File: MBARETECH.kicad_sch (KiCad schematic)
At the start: 48 parts, among them J10 Conn_01x03, J11 Conn_01x03, J17 Conn_01x03, J18 Conn_01x03, J19 TERMINAL DRIVER, J3 XT60-M, J7 Conn_01x03, J8 Conn_01x03, J9 Conn_01x03, SW1 SW_SPDT, SW2 SW_DIP_x04, SW3 SW_SPDT, SW5 SW_SPST, U2 ESP32-S3-DevKitC

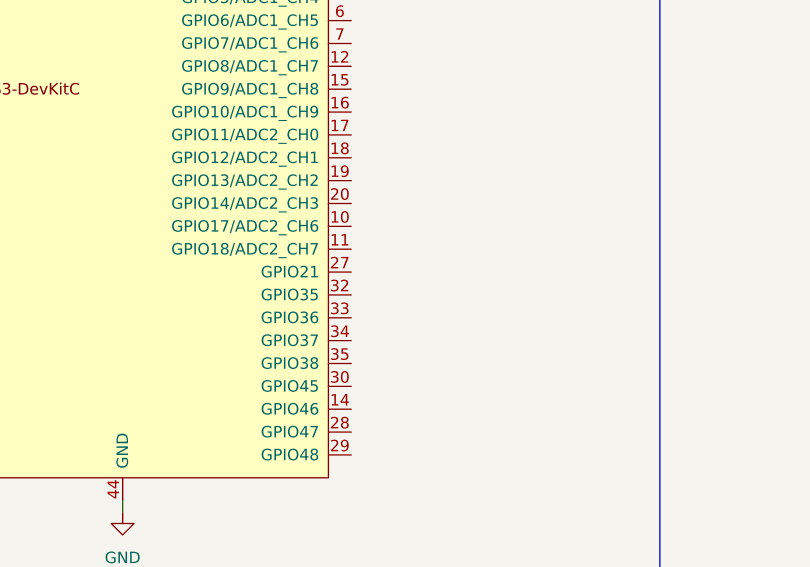
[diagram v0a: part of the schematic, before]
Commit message: test branch
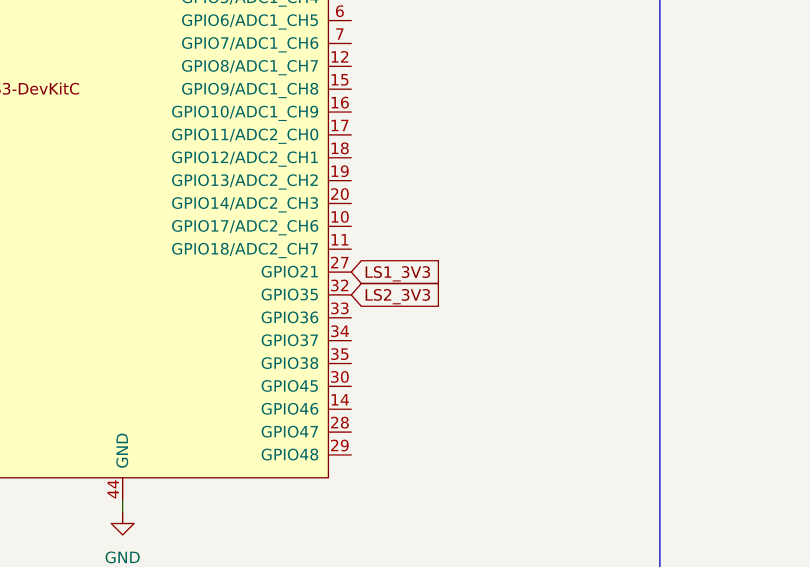
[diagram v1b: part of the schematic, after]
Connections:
- net LS1_3V3: now also U2.27 (GPIO21)
- net LS2_3V3: now also U2.32 (GPIO35)
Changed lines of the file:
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@@
+		)
+	)
+	(global_label "LS1_3V3"
+		(shape input)
+		(at 111.76 110.49 0)
+		(fields_autoplaced yes)
+		(effects
+			(font
+				(size 1.27 1.27)
+			)
+			(justify left)
+		)
+		(property "Intersheetrefs" "${INTERSHEET_REFS}"
+			(at 122.6675 110.49 0)
+			(effects
+				(font
+					(size 1.27 1.27)
+				)
+				(justify left)
+				(hide yes)
+			)
+		)
+	)
+	(global_label "LS2_3V3"
+		(shape input)
+		(at 111.76 113.03 0)
+		(fields_autoplaced yes)
+		(effects
+			(font
+				(size 1.27 1.27)
+			)
+			(justify left)
+		)
+		(property "Intersheetrefs" "${INTERSHEET_REFS}"
+			(at 122.6675 113.03 0)
+			(effects
+				(font
+					(size 1.27 1.27)
+				)
+				(justify left)
+				(hide yes)
+			)
 		)
 	)

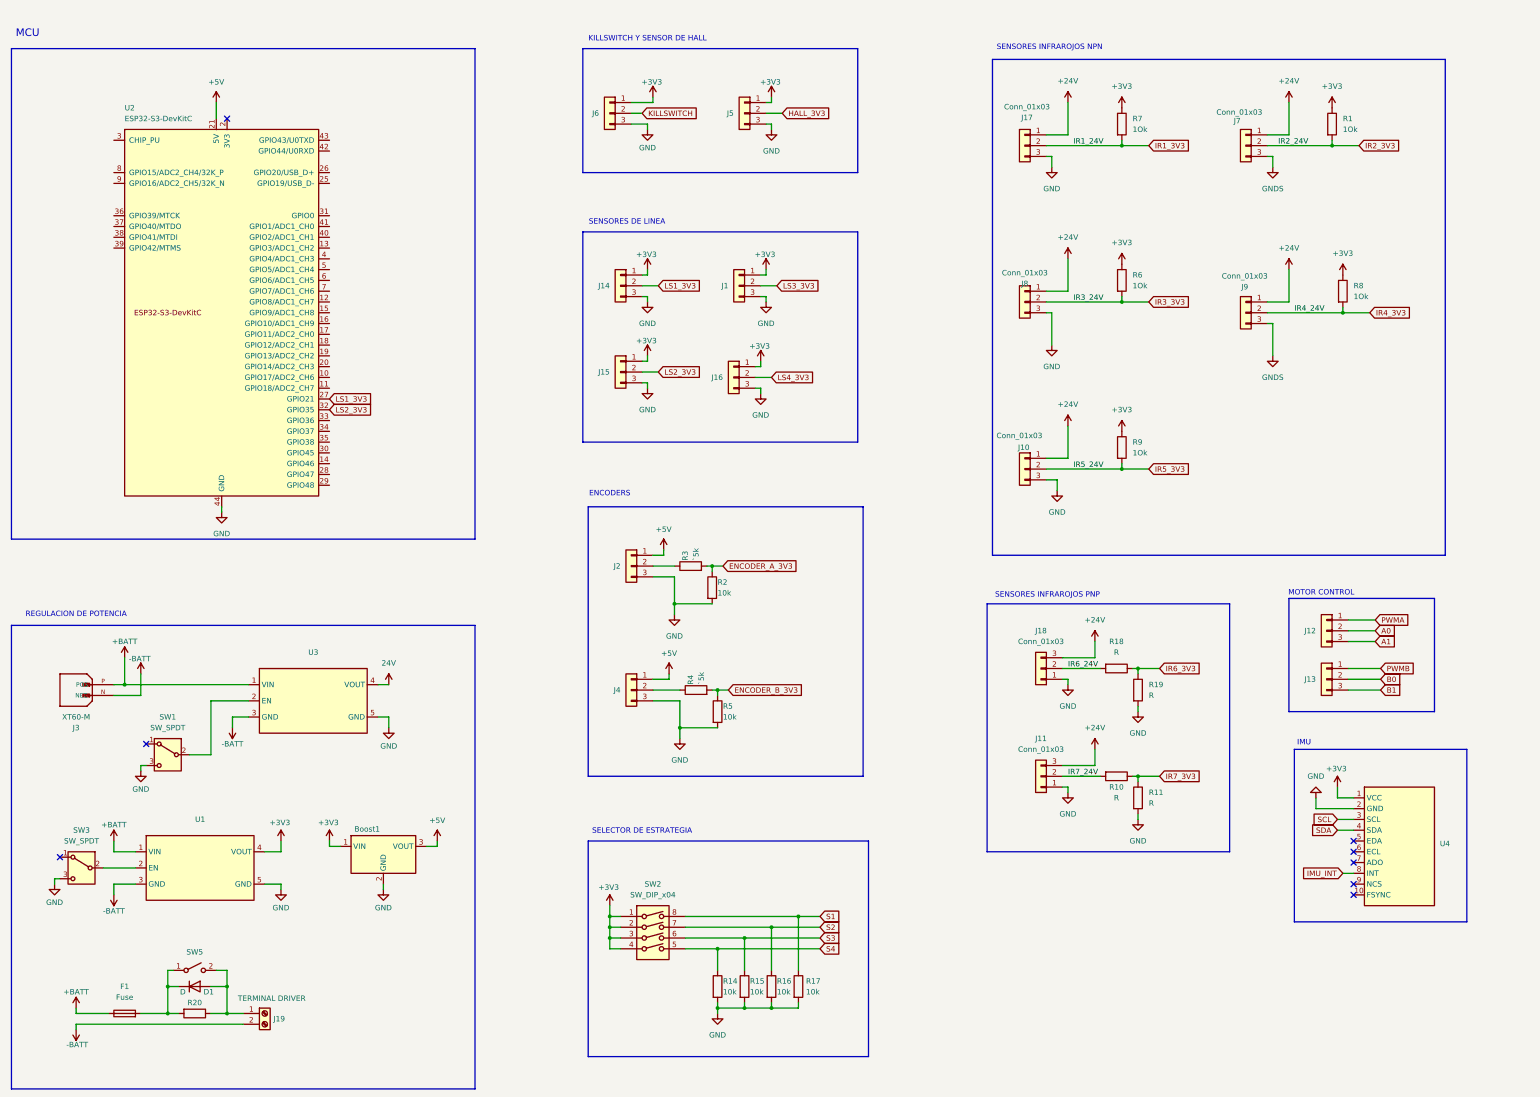
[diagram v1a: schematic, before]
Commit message: Version final
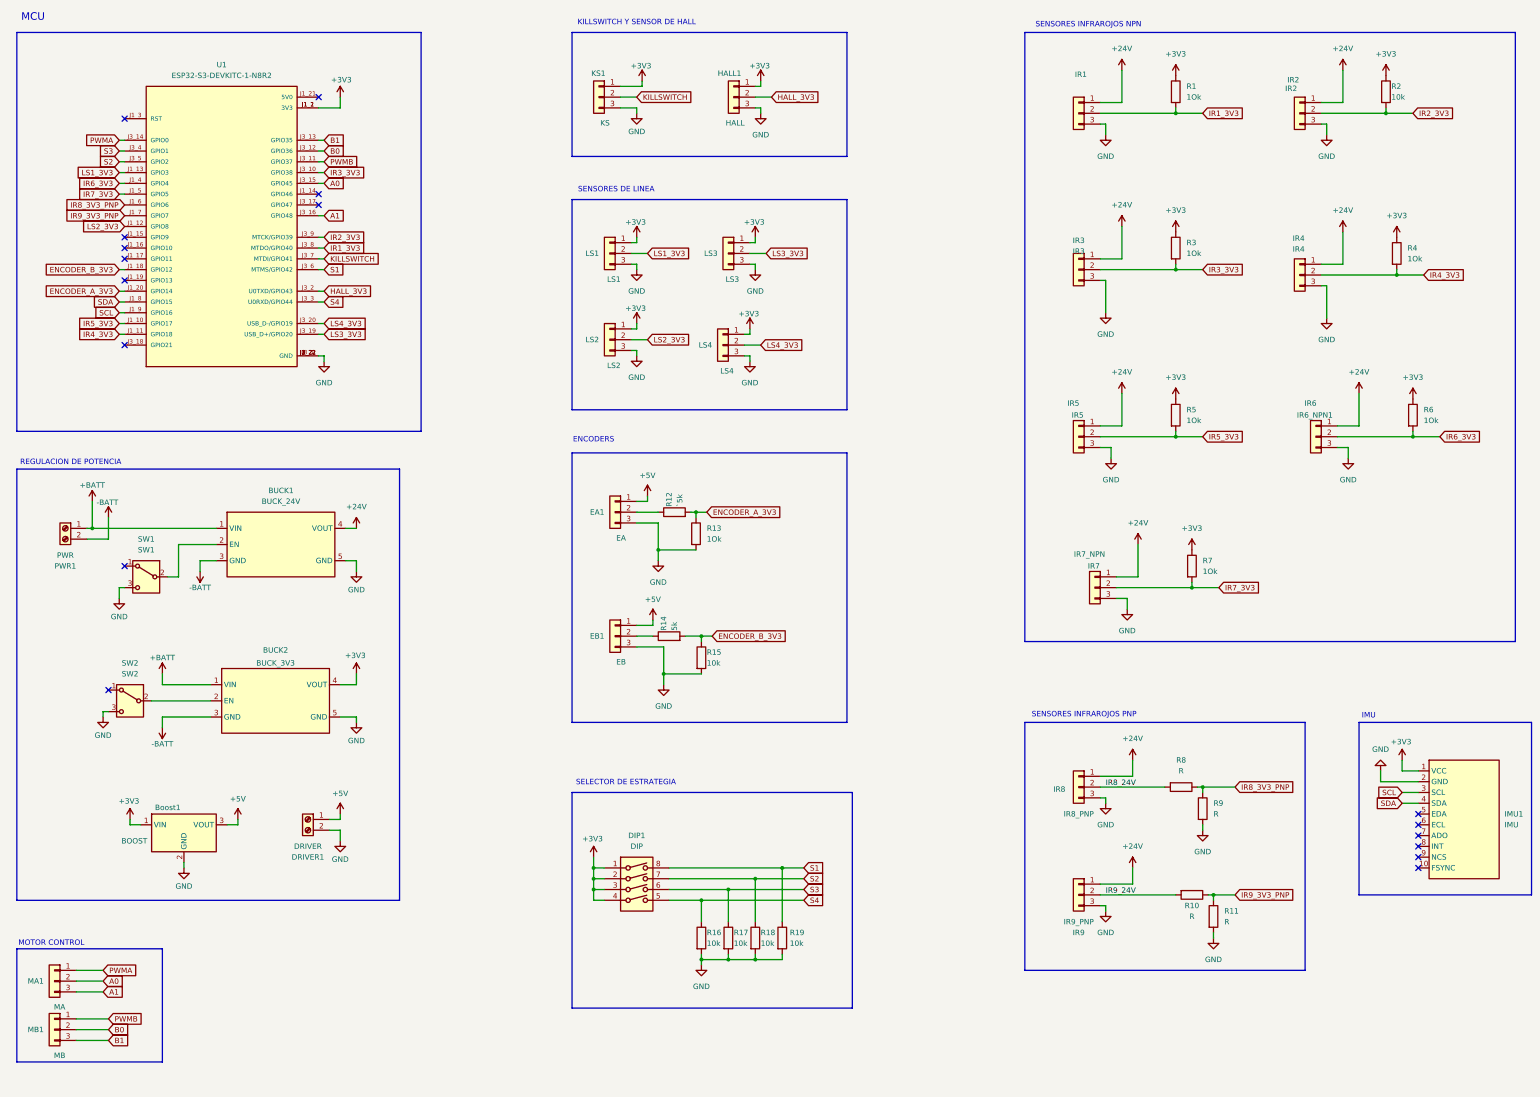
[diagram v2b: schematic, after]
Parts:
- removed D1: D, symbol Device:D
- removed F1: Fuse, symbol Device:Fuse
- removed J19: TERMINAL DRIVER, symbol Connector:Screw_Terminal_01x02
- removed J3: XT60-M, XT60-M:AMASS_XT60-M, symbol XT60-M:XT60-M
- removed R20: R, symbol Device:R
- removed SW5: SW_SPST, symbol Switch:SW_SPST
- removed U2: ESP32-S3-DevKitC, PCM_Espressif:ESP32-S3-DevKitC, symbol Espressif:ESP32-S3-DevKitC
- added DRIVER1: DRIVER, TerminalBlock_Phoenix:TerminalBlock_Phoenix_MKDS-1,5-2-5.08_1x02_P5.08mm_Horizontal, symbol Connector:Screw_Terminal_01x02
- added IR6_NPN1: IR6, Connector_JST:JST_XH_B3B-XH-A_1x03_P2.50mm_Vertical, symbol Connector_Generic:Conn_01x03
- added IR7: IR7_NPN, Connector_JST:JST_XH_B3B-XH-A_1x03_P2.50mm_Vertical, symbol Connector_Generic:Conn_01x03
- added PWR1: PWR, TerminalBlock_Phoenix:TerminalBlock_Phoenix_MKDS-1,5-2-5.08_1x02_P5.08mm_Horizontal, symbol Connector:Screw_Terminal_01x02
- added R6, R7: 1Ok, Resistor_SMD:R_0603_1608Metric_Pad0.98x0.95mm_HandSolder, symbol Device:R
- added U1: ESP32-S3-DEVKITC-1-N8R2, ESP32-S3-DEVKITC-1-N8R2:XCVR_ESP32-S3-DEVKITC-1-N8R2, symbol ESP32-S3-DEVKITC-1-N8R2:ESP32-S3-DEVKITC-1-N8R2
- BUCK1: renamed from U3; value ~ -> BUCK_24V; footprint (none) -> Mbaretech_buckConverter:Buck-Converter
- BUCK2: renamed from U1; value ~ -> BUCK_3V3; footprint (none) -> Mbaretech_buckConverter:Buck-Converter
- Boost1: value ~ -> BOOST; footprint (none) -> Connector_PinHeader_2.54mm:PinHeader_1x03_P2.54mm_Vertical
- DIP1: renamed from SW2; value SW_DIP_x04 -> DIP; footprint (none) -> Button_Switch_THT:SW_DIP_SPSTx04_Slide_9.78x12.34mm_W7.62mm_P2.54mm
- EA1: renamed from J2; value ~ -> EA; footprint Connector_JST:JST_PH_B9B-PH-K_1x09_P2.00mm_Vertical -> Connector_JST:JST_XH_B3B-XH-A_1x03_P2.50mm_Vertical
- EB1: renamed from J4; value ~ -> EB; footprint Connector_JST:JST_PH_B9B-PH-K_1x09_P2.00mm_Vertical -> Connector_JST:JST_XH_B3B-XH-A_1x03_P2.50mm_Vertical
- HALL1: renamed from J5; value ~ -> HALL; footprint Connector_JST:JST_PH_B9B-PH-K_1x09_P2.00mm_Vertical -> Connector_JST:JST_XH_B3B-XH-A_1x03_P2.50mm_Vertical
- IMU1: renamed from U4; value ~ -> IMU; footprint (none) -> Connector_PinHeader_2.54mm:PinHeader_1x10_P2.54mm_Vertical
- IR1: renamed from J17; value Conn_01x03 -> IR1; footprint Connector_AMASS:AMASS_XT60-F_1x02_P7.20mm_Vertical -> Connector_JST:JST_XH_B3B-XH-A_1x03_P2.50mm_Vertical
- IR2: renamed from J7; value Conn_01x03 -> IR2; footprint Connector_AMASS:AMASS_XT60-F_1x02_P7.20mm_Vertical -> Connector_JST:JST_XH_B3B-XH-A_1x03_P2.50mm_Vertical
- IR3: renamed from J8; value Conn_01x03 -> IR3; footprint Connector_AMASS:AMASS_XT60-F_1x02_P7.20mm_Vertical -> Connector_JST:JST_XH_B3B-XH-A_1x03_P2.50mm_Vertical
- IR4: renamed from J9; value Conn_01x03 -> IR4; footprint Connector_AMASS:AMASS_XT60-F_1x02_P7.20mm_Vertical -> Connector_JST:JST_XH_B3B-XH-A_1x03_P2.50mm_Vertical
- IR5: renamed from J10; value Conn_01x03 -> IR5; footprint Connector_AMASS:AMASS_XT60-F_1x02_P7.20mm_Vertical -> Connector_JST:JST_XH_B3B-XH-A_1x03_P2.50mm_Vertical
- IR8: renamed from J18; value Conn_01x03 -> IR8_PNP; footprint Connector_AMASS:AMASS_XT60-F_1x02_P7.20mm_Vertical -> Connector_JST:JST_XH_B3B-XH-A_1x03_P2.50mm_Vertical
- IR9: renamed from J11; value Conn_01x03 -> IR9_PNP; footprint Connector_AMASS:AMASS_XT60-F_1x02_P7.20mm_Vertical -> Connector_JST:JST_XH_B3B-XH-A_1x03_P2.50mm_Vertical
- KS1: renamed from J6; value ~ -> KS; footprint Connector_JST:JST_PH_B9B-PH-K_1x09_P2.00mm_Vertical -> Connector_JST:JST_XH_B3B-XH-A_1x03_P2.50mm_Vertical
- LS1: renamed from J14; value ~ -> LS1; footprint Connector_JST:JST_PH_B9B-PH-K_1x09_P2.00mm_Vertical -> Connector_JST:JST_XH_B3B-XH-A_1x03_P2.50mm_Vertical
- LS2: renamed from J15; value ~ -> LS2; footprint Connector_JST:JST_PH_B9B-PH-K_1x09_P2.00mm_Vertical -> Connector_JST:JST_XH_B3B-XH-A_1x03_P2.50mm_Vertical
- LS3: renamed from J1; value ~ -> LS3; footprint Connector_JST:JST_PH_B9B-PH-K_1x09_P2.00mm_Vertical -> Connector_JST:JST_XH_B3B-XH-A_1x03_P2.50mm_Vertical
- LS4: renamed from J16; value ~ -> LS4; footprint Connector_JST:JST_PH_B9B-PH-K_1x09_P2.00mm_Vertical -> Connector_JST:JST_XH_B3B-XH-A_1x03_P2.50mm_Vertical
- MA1: renamed from J12; value ~ -> MA; footprint Connector_JST:JST_PH_B9B-PH-K_1x09_P2.00mm_Vertical -> Connector_JST:JST_XH_B3B-XH-A_1x03_P2.50mm_Vertical
- MB1: renamed from J13; value ~ -> MB; footprint Connector_JST:JST_PH_B9B-PH-K_1x09_P2.00mm_Vertical -> Connector_JST:JST_XH_B3B-XH-A_1x03_P2.50mm_Vertical
- R1, R10, R11, R2: footprint (none) -> Resistor_SMD:R_0603_1608Metric_Pad0.98x0.95mm_HandSolder
- R12: renamed from R3; footprint (none) -> Resistor_SMD:R_0603_1608Metric_Pad0.98x0.95mm_HandSolder
- R13: renamed from R7; footprint (none) -> Resistor_SMD:R_0603_1608Metric_Pad0.98x0.95mm_HandSolder
- R14: renamed from R4; value `5k -> 5k; footprint (none) -> Resistor_SMD:R_0603_1608Metric_Pad0.98x0.95mm_HandSolder
- R15: renamed from R5; footprint (none) -> Resistor_SMD:R_0603_1608Metric_Pad0.98x0.95mm_HandSolder
- R16: renamed from R14; footprint (none) -> Resistor_SMD:R_0603_1608Metric_Pad0.98x0.95mm_HandSolder
- R17: renamed from R15; footprint (none) -> Resistor_SMD:R_0603_1608Metric_Pad0.98x0.95mm_HandSolder
- R18: renamed from R16; footprint (none) -> Resistor_SMD:R_0603_1608Metric_Pad0.98x0.95mm_HandSolder
- R19: renamed from R17; footprint (none) -> Resistor_SMD:R_0603_1608Metric_Pad0.98x0.95mm_HandSolder
- R3: renamed from R6; footprint (none) -> Resistor_SMD:R_0603_1608Metric_Pad0.98x0.95mm_HandSolder
- R4: renamed from R8; footprint (none) -> Resistor_SMD:R_0603_1608Metric_Pad0.98x0.95mm_HandSolder
- R5: renamed from R9; footprint (none) -> Resistor_SMD:R_0603_1608Metric_Pad0.98x0.95mm_HandSolder
- R8: renamed from R18; footprint (none) -> Resistor_SMD:R_0603_1608Metric_Pad0.98x0.95mm_HandSolder
- R9: renamed from R19; footprint (none) -> Resistor_SMD:R_0603_1608Metric_Pad0.98x0.95mm_HandSolder
- SW1: value SW_SPDT -> SW1; footprint (none) -> SPDT_SlideSwitch:tht
- SW2: renamed from SW3; value SW_SPDT -> SW2; footprint (none) -> SPDT_SlideSwitch:tht
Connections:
- net 24V is gone; now on net +24V: BUCK1.4 (VOUT)
- net GNDS is gone; now on net GND: IR2.3 (Pin_3), IR4.3 (Pin_3)
- net +24V: now also IR8.1 (Pin_1), IR9.1 (Pin_1), IR6_NPN1.1 (Pin_1), IR7.1 (Pin_1); no longer IR8.3 (Pin_3), IR9.3 (Pin_3)
- net +3V3: now also R2.1, R6.1, R7.1, U1.J1_1 (3V3), U1.J1_2 (3V3); no longer R13.1
- net +5V: now also DRIVER1.1 (Pin_1)
- net +BATT: now also PWR1.1 (Pin_1)
- net -BATT: now also PWR1.2 (Pin_2)
- net A0: now also U1.J3_15 (GPIO45)
- net A1: now also U1.J3_16 (GPIO48)
- net B0: now also U1.J3_12 (GPIO36)
- net B1: now also U1.J3_13 (GPIO35)
- net ENCODER_A_3V3: now also R13.1, U1.J1_20 (GPIO14); no longer R2.1
- net ENCODER_B_3V3: now also U1.J1_18 (GPIO12)
- net GND: now also IR8.3 (Pin_3), IR9.3 (Pin_3), R13.2, DRIVER1.2 (Pin_2), IR6_NPN1.3 (Pin_3), IR7.3 (Pin_3), U1.J1_22 (GND), U1.J3_1 (GND), U1.J3_21 (GND), U1.J3_22 (GND); no longer IR8.1 (Pin_1), IR9.1 (Pin_1), R2.2
- net HALL_3V3: now also U1.J3_2 (U0TXD/GPIO43)
- net IR1_3V3: now also R1.2, U1.J3_8 (MTDO/GPIO40); no longer R13.2
- net IR2_3V3: now also R2.2, U1.J3_9 (MTCK/GPIO39); no longer R1.2
- net IR3_3V3: now also U1.J3_10 (GPIO38)
- net IR4_3V3: now also U1.J1_11 (GPIO18)
- net IR5_3V3: now also U1.J1_10 (GPIO17)
- net IR6_3V3: now also IR6_NPN1.2 (Pin_2), R6.2, U1.J1_4 (GPIO4); no longer R8.1, R9.1
- net IR7_3V3: now also IR7.2 (Pin_2), R7.2, U1.J1_5 (GPIO5); no longer R10.1, R11.1
- net KILLSWITCH: now also U1.J3_7 (MTDI/GPIO41)
- net LS1_3V3: now also U1.J1_13 (GPIO3)
- net LS2_3V3: now also U1.J1_12 (GPIO8)
- net LS3_3V3: now also U1.J3_19 (USB_D+/GPIO20)
- net LS4_3V3: now also U1.J3_20 (USB_D-/GPIO19)
- net PWMA: now also U1.J3_14 (GPIO0)
- net PWMB: now also U1.J3_11 (GPIO37)
- net S1: now also U1.J3_6 (MTMS/GPIO42)
- net S2: now also U1.J3_5 (GPIO2)
- net S3: now also U1.J3_4 (GPIO1)
- net S4: now also U1.J3_3 (U0RXD/GPIO44)
- net SCL: now also U1.J1_9 (GPIO16)
- net SDA: now also U1.J1_8 (GPIO15)
- net IMU_INT: no longer names the net of IMU1.8 (INT)
- net IR6_24V renamed IR8_24V
- net IR7_24V renamed IR9_24V
- new net IR8_3V3_PNP: R8.1, R9.1, U1.J1_6 (GPIO6)
- new net IR9_3V3_PNP: R10.1, R11.1, U1.J1_7 (GPIO7)
- no-connect marks 8 -> 17
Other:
- moved on the sheet: BUCK1, BUCK2, Boost1, DIP1, EA1, EB1, HALL1, IMU1, IR2, IR3, IR4, IR5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
